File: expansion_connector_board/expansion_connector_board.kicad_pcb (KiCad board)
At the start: 2 copper layers, 139 x 89 mm, 6 parts, among them J1 Conn_01x04, J12 Conn_02x17_Top_Bottom, J13 Conn_01x04, J3 Conn_02x17_Top_Bottom

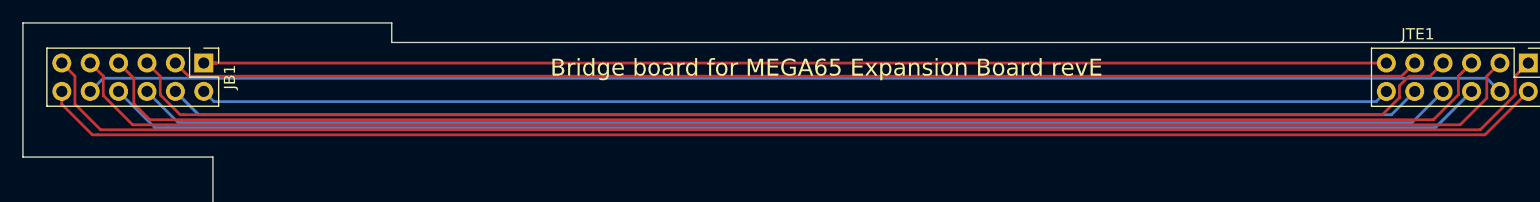
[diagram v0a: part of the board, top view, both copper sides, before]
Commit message: work on various checking various measurements
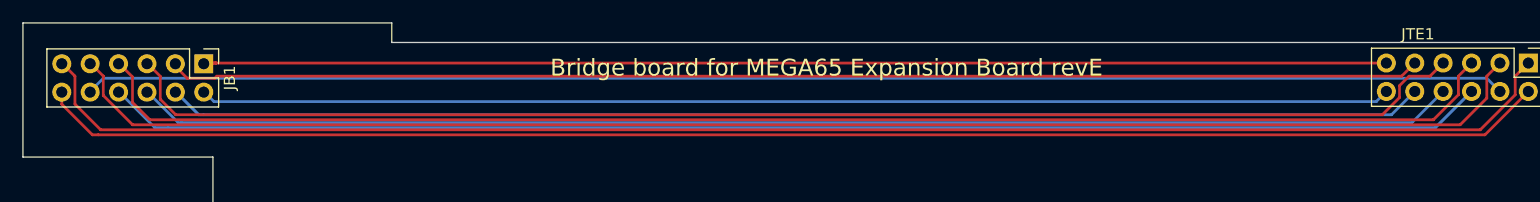
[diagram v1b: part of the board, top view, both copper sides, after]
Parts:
- moved JB1 0.07 mm to (73.2, 38.7)
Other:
- board text added: "H4 is here"
- board text added: "Left PMOD on MEGA65 Board"
- board text added: "Left PMOD on expansion board"
